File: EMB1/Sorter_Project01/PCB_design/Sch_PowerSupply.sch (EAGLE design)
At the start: 13 parts, among them IC1 LM2574N-3.3, IC2 7812T, IC3 7806T

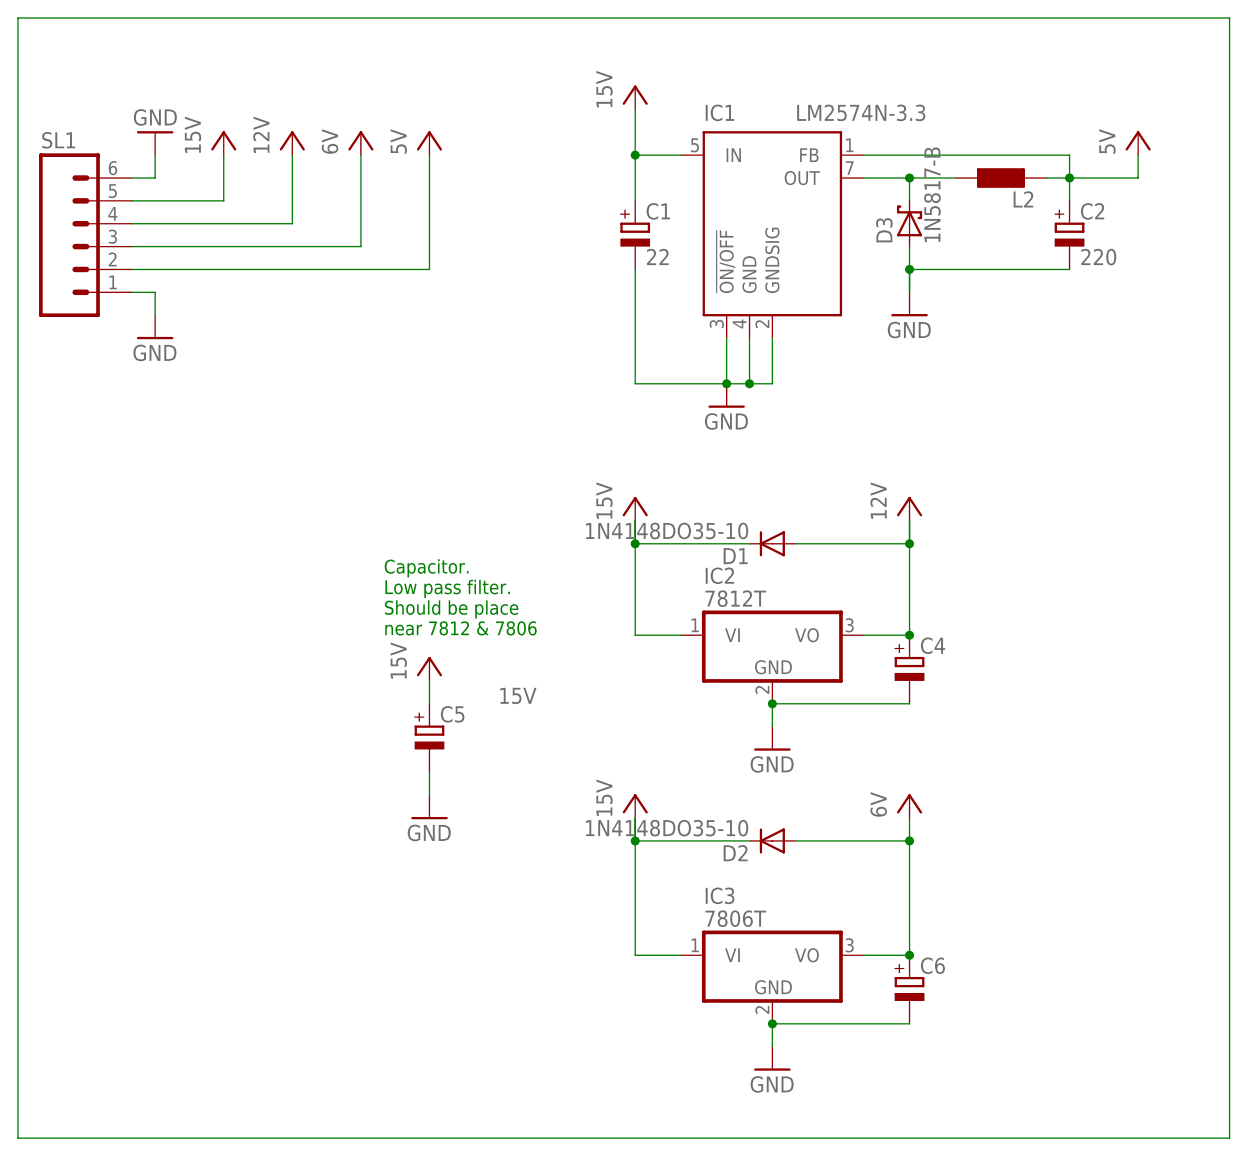
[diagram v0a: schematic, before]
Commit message: report images added
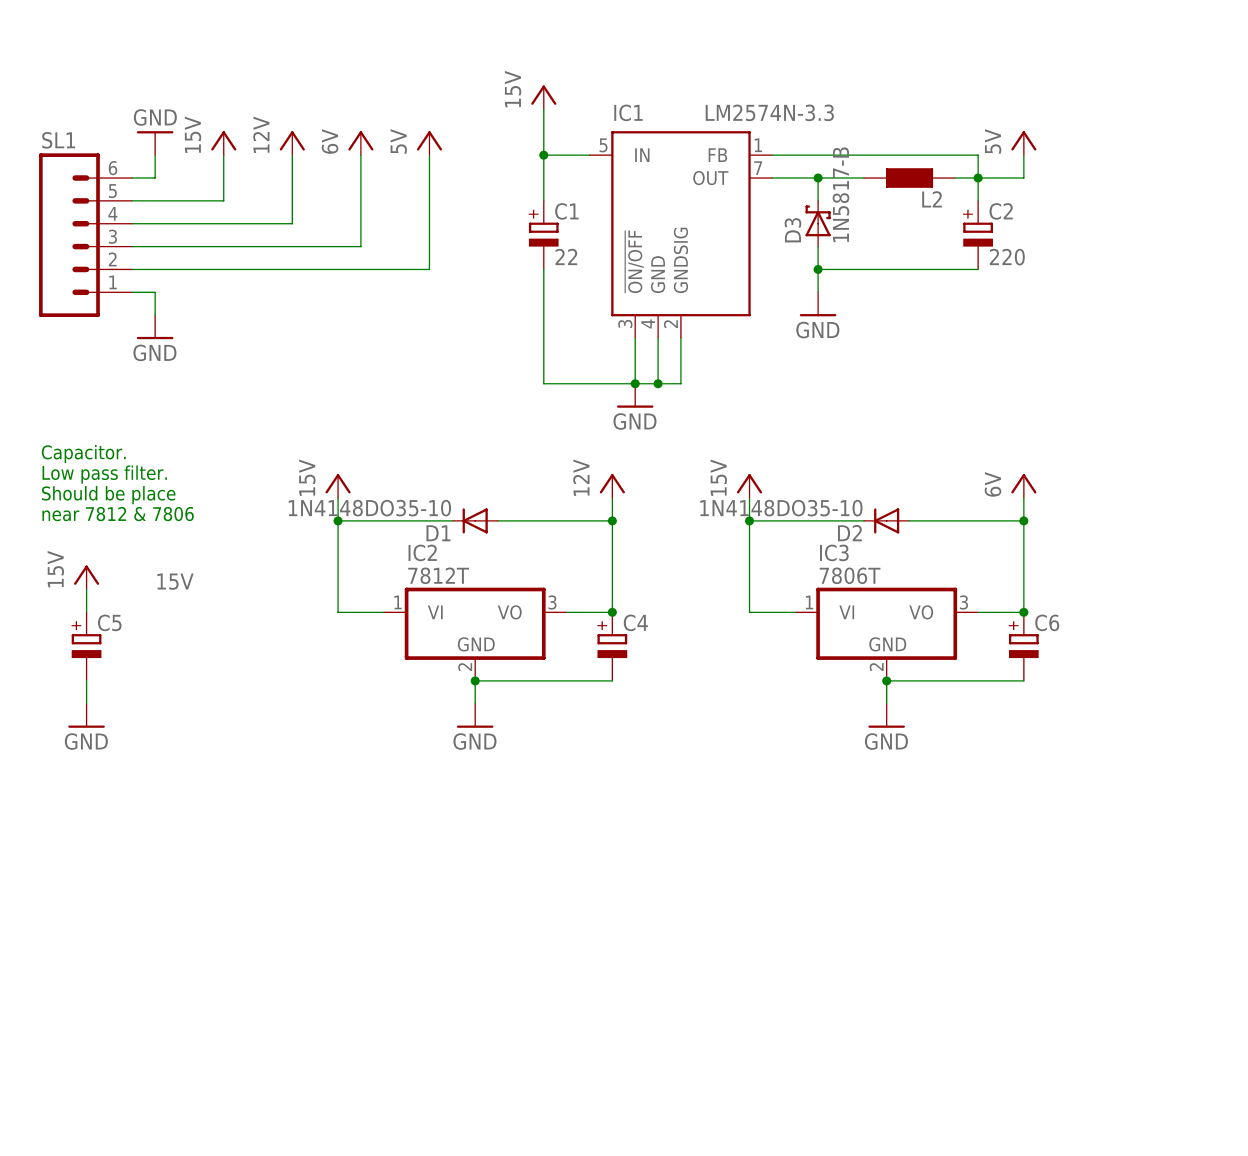
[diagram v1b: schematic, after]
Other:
- moved on the sheet: C1, C2, C4, C5, C6, D1, D2, D3, IC1, IC2, IC3, L2
